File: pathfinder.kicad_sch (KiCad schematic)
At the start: 2 parts, among them SW1 SW_Push, U1 XIAO-RP2040-DIP

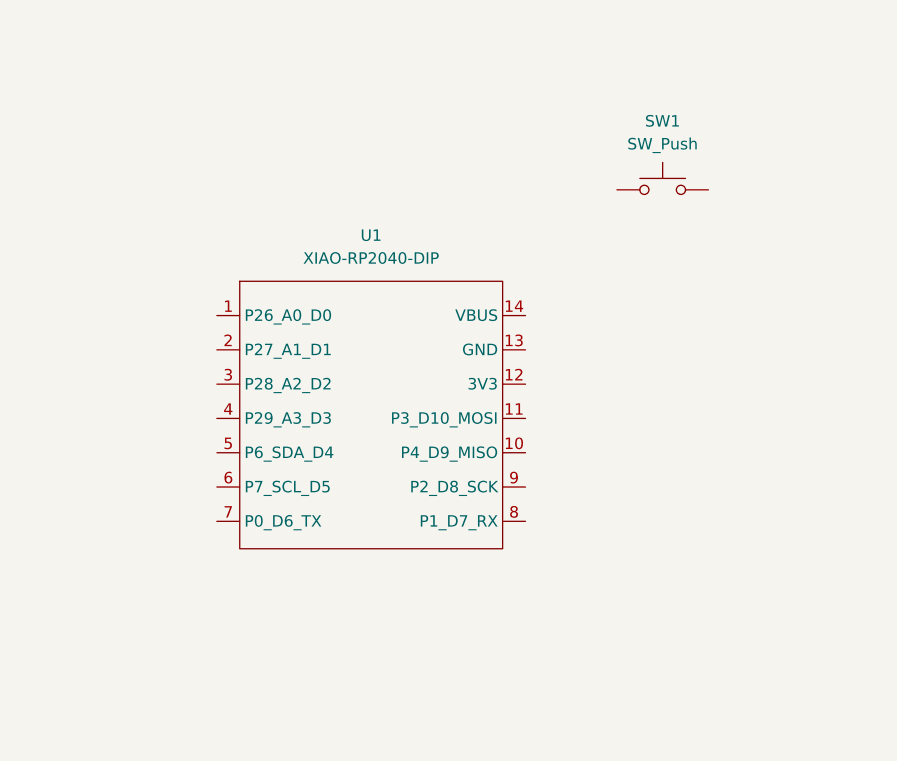
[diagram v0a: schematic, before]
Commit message: dump
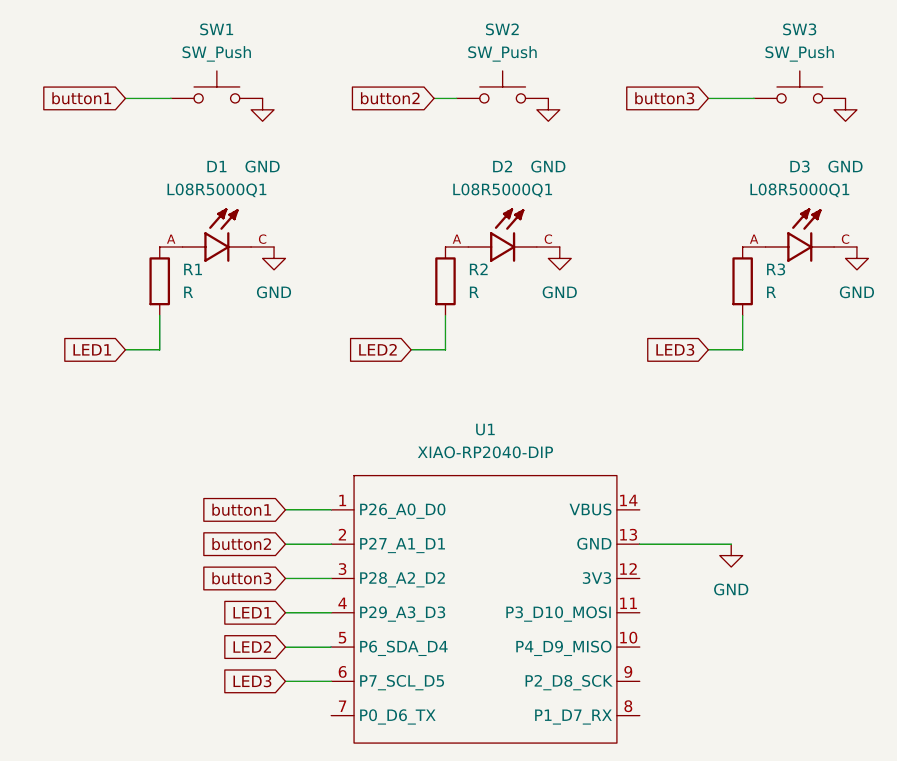
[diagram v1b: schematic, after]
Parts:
- added D1, D2, D3: L08R5000Q1, L08R5000Q1:LEDRD254W57D500H1070, symbol L08R5000Q1:L08R5000Q1
- added R1, R2, R3: R, symbol Device:R
- added SW2, SW3: SW_Push, symbol Switch:SW_Push
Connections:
- net button1: now reaches SW1.1
- net button1: now also U1.1 (P26_A0_D0)
- net GND: now reaches SW1.2
- net GND: now also U1.13 (GND), D1.C, D2.C, D3.C, SW2.2, SW3.2
- net button2: now reaches U1.2 (P27_A1_D1)
- net button2: now also SW2.1
- net button3: now reaches U1.3 (P28_A2_D2)
- net button3: now also SW3.1
- net LED1: now reaches U1.4 (P29_A3_D3)
- net LED1: now also R1.2
- net LED2: now reaches U1.5 (P6_SDA_D4)
- net LED2: now also R2.2
- net LED3: now reaches U1.6 (P7_SCL_D5)
- net LED3: now also R3.2
- new net: D2.A, R2.1
- new net: D3.A, R3.1
- new net: D1.A, R1.1
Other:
- moved on the sheet: SW1, U1
